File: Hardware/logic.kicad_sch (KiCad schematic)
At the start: 78 parts, among them J301 Ref Divider, J302 GPS ANT, J303 Encoder, J304 Ref Select, J305 Ref Range, J306 GPS Module, J308 RF 50 Ohm, J309 RF TTL, J310 1PPS TTL, J311 ICSP, J312 Serial, J313 Program, J314 LCD, Q301 2N3904, U301 DAC8571IDGK, U302 NEO-M8M, U303 OP07, U304 OP07, U305 TXS0108EPW, U306 GALI-52, U307 74LVC1G17, U308 74LVC1G17, U309 MCP23017_SO, U310 MAX232, U311 PIC18F27Q43, U312 24AA04

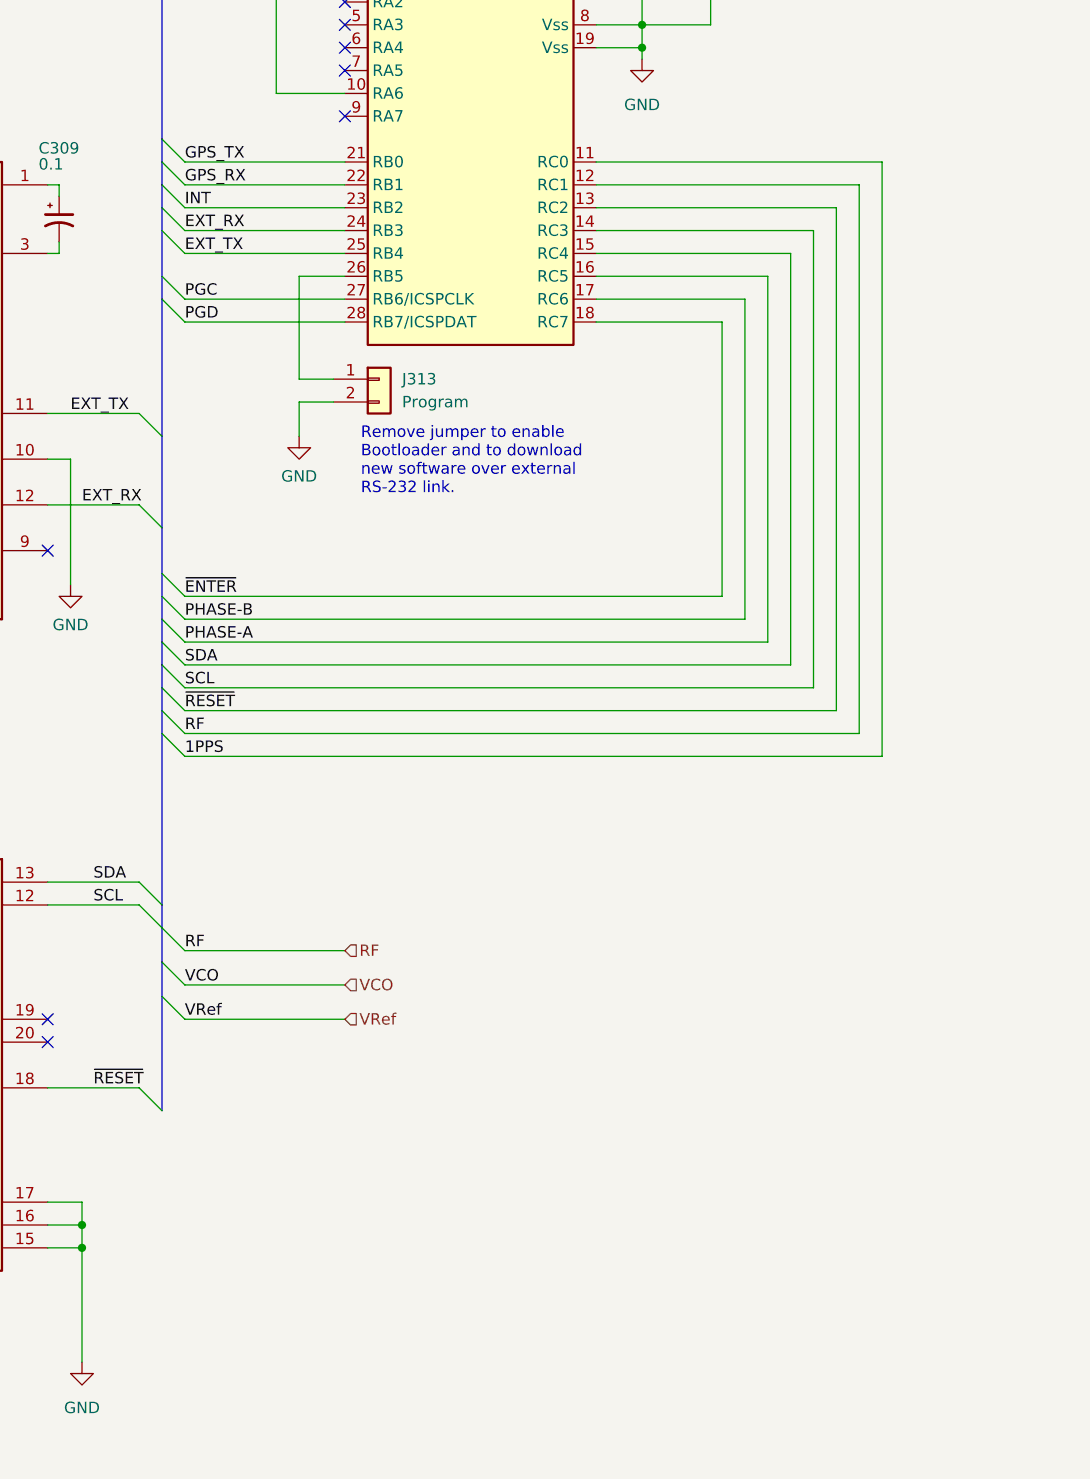
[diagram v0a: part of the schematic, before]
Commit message: updated gps serial
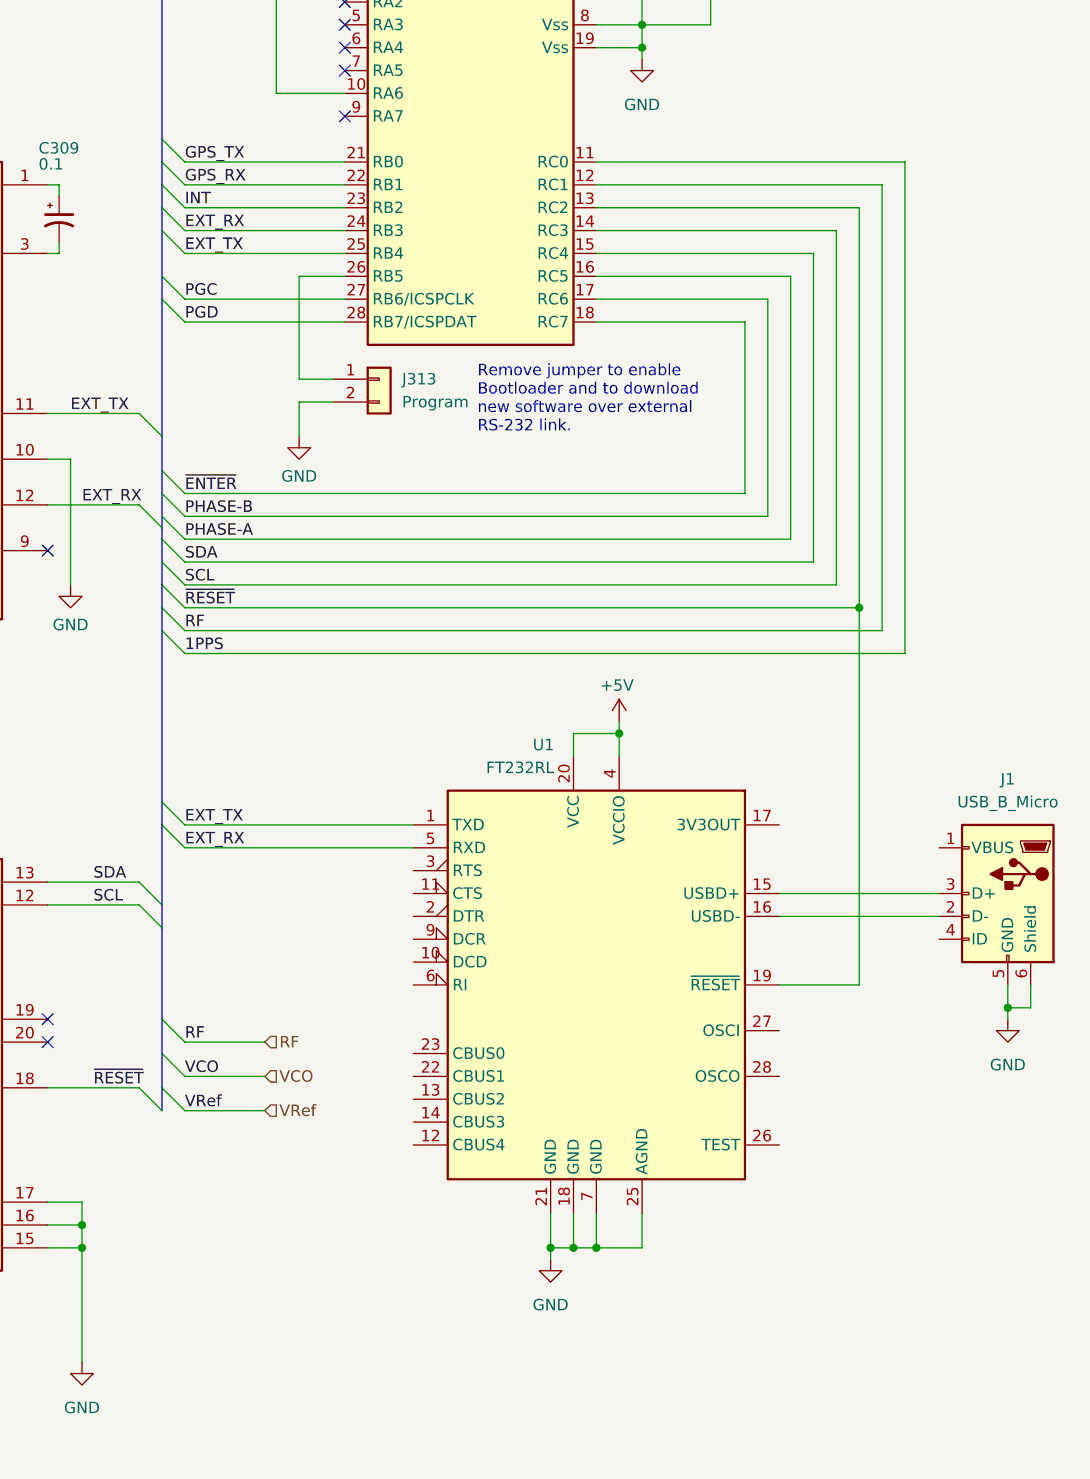
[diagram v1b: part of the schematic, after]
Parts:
- added J1: USB_B_Micro, symbol Connector:USB_B_Micro
- added U1: FT232RL, Package_SO:SSOP-28_5.3x10.2mm_P0.65mm, symbol Interface_USB:FT232RL
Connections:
- net +5V: now also U1.20 (VCC), U1.4 (VCCIO)
- net EXT_RX: now also U1.5 (RXD)
- net EXT_TX: now also U1.1 (TXD)
- net GND: now also J1.5 (GND), J1.6 (Shield), U1.18 (GND), U1.21 (GND), U1.25 (AGND), U1.7 (GND)
- net ~{RESET}: now also U1.19 (~{RESET})
- new net: J1.2 (D-), U1.16 (USBD-)
- new net: J1.3 (D+), U1.15 (USBD+)
